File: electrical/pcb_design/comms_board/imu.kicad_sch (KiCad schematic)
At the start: 19 parts, among them U2 BMI323, U3 BMI323

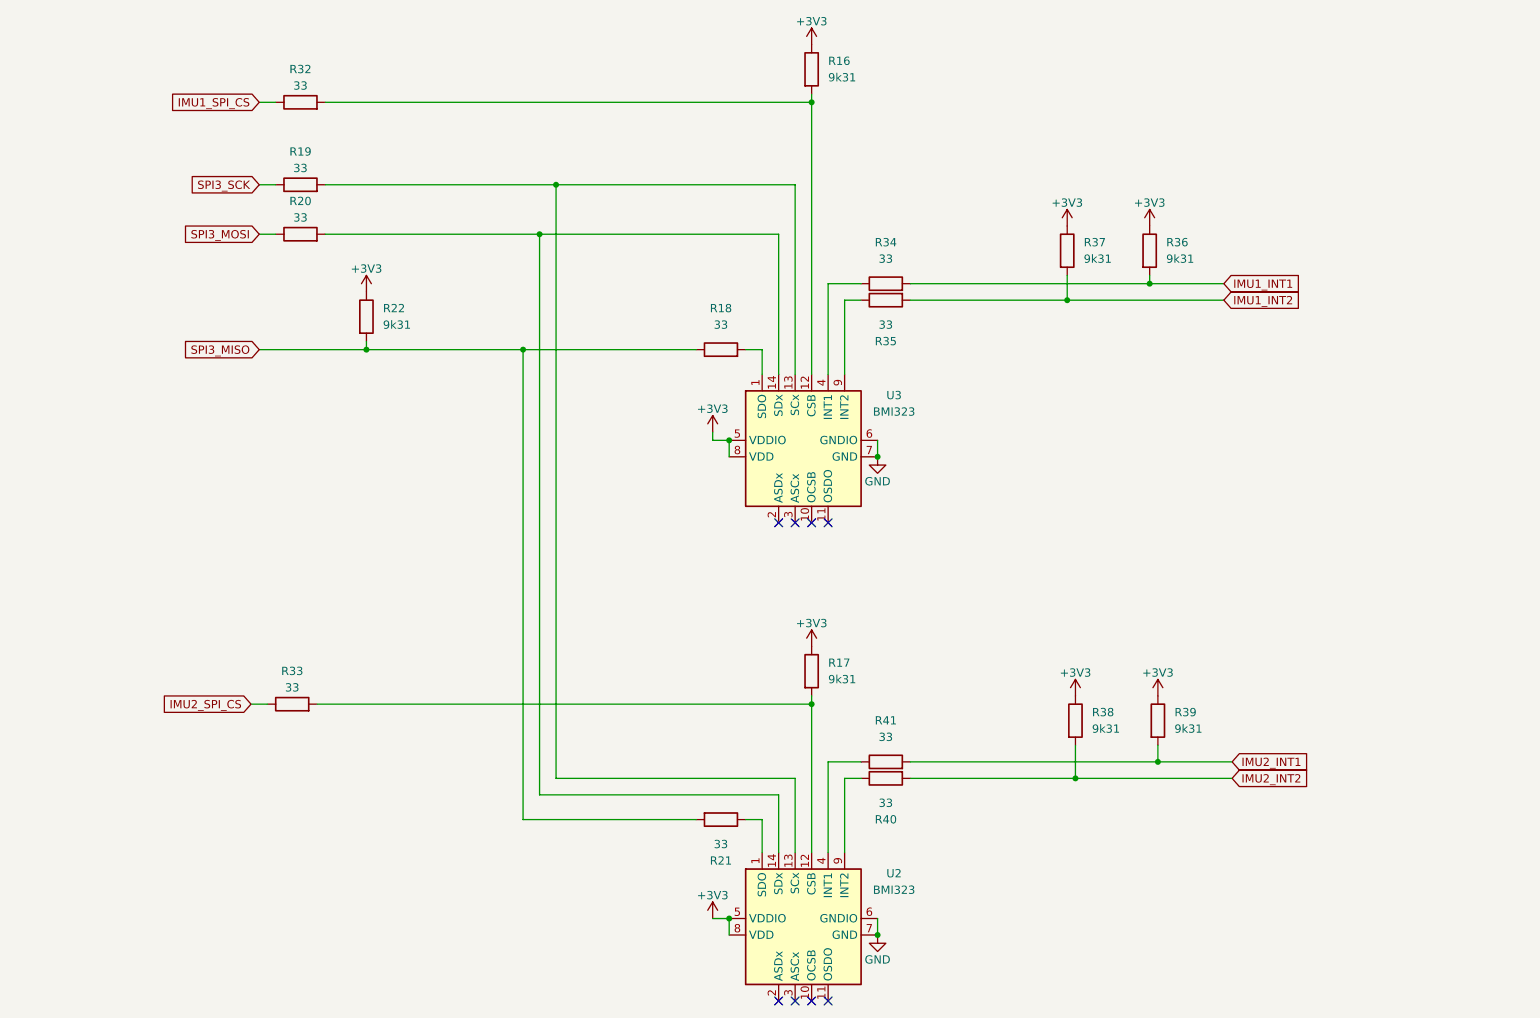
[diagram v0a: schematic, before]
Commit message: First draft of Cheerful Coffee comms board
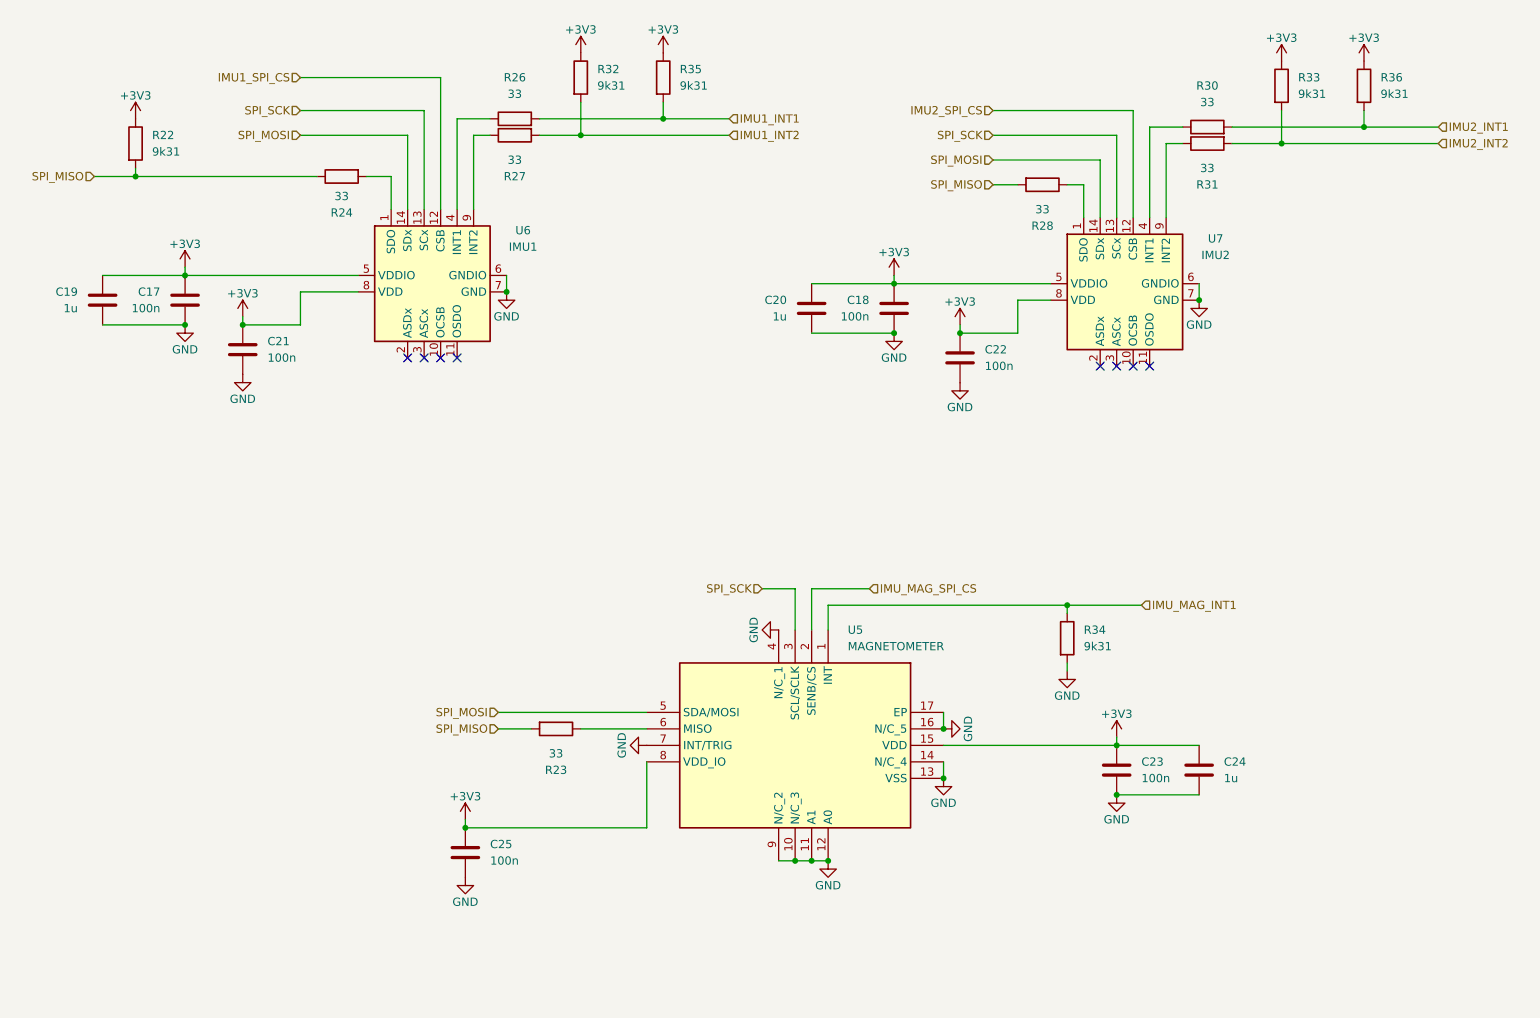
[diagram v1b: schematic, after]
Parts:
- removed R16, R17: 9k31, footprints:Nondescript_R_0402_1005Metric, symbol Device:R
- removed R19, R20, R32, R33: 33, footprints:Nondescript_R_0402_1005Metric, symbol Device:R
- added C17, C18, C21, C22, C23, C25: 100n, footprints:Nondescript_C_0402_1005Metric, symbol Device:C
- added C19, C20, C24: 1u, footprints:Nondescript_C_0402_1005Metric, symbol Device:C
- added R23: 33, footprints:Nondescript_R_0402_1005Metric, symbol Device:R
- added R34: 9k31, footprints:Nondescript_R_0402_1005Metric, symbol Device:R
- added U5: MAGNETOMETER, footprints:QFN50P300X300X100-17N-D, symbol TVSC:MLX90393ELW-ABA-011-RE
- U6: renamed from U3; value BMI323 -> IMU1
- U7: renamed from U2; value BMI323 -> IMU2
- renumbered R18 to R24, R34 to R26, R35 to R27, R21 to R28, R41 to R30, R40 to R31, R37 to R32, R38 to R33, R36 to R35, R39 to R36
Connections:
- net +3V3: now also C17.1, C18.1, C19.1, C20.1, C21.1, C22.1, C23.1, C24.1, C25.1, U5.15 (VDD), U5.8 (VDD_IO)
- net GND: now also C17.2, C18.2, C19.2, C20.2, C21.2, C22.2, C23.2, C24.2, C25.2, R34.2, U5.10 (N/C_3), U5.11 (A1), U5.12 (A0), U5.13 (VSS), U5.14 (N/C_4), U5.16 (N/C_5), U5.17 (EP), U5.4 (N/C_1), U5.7 (INT/TRIG), U5.9 (N/C_2)
- net IMU1_SPI_CS: now also U6.12 (CSB)
- net IMU2_SPI_CS: now also U7.12 (CSB)
- net SPI_SCK: now reaches U6.13 (SCx), U7.13 (SCx)
- net SPI_SCK: now also U5.3 (SCL/SCLK)
- net SPI_MOSI: now reaches U6.14 (SDx), U7.14 (SDx)
- net SPI_MOSI: now also U5.5 (SDA/MOSI)
- net SPI3_MISO renamed SPI_MISO
- net SPI_MISO: now also R23.2
- new net: R23.1, U5.6 (MISO)
- new net IMU_MAG_INT1: R34.1, U5.1 (INT)
- new net IMU_MAG_SPI_CS: U5.2 (SENB/CS)
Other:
- moved on the sheet: R22, R24, R26, R27, R28, R30, R31, R32, R33, R35, R36, U6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
